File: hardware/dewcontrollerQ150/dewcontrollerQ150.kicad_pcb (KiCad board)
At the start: 2 copper layers, 54.1 x 52 mm, 17 parts, among them J1 12V Power, J2 Dew Heater, J3 SHT45 Sensor, Q1 FQP 30N06L, U2 Buck_12V_5V, U3 XIAO-ESP32-S3-DIP

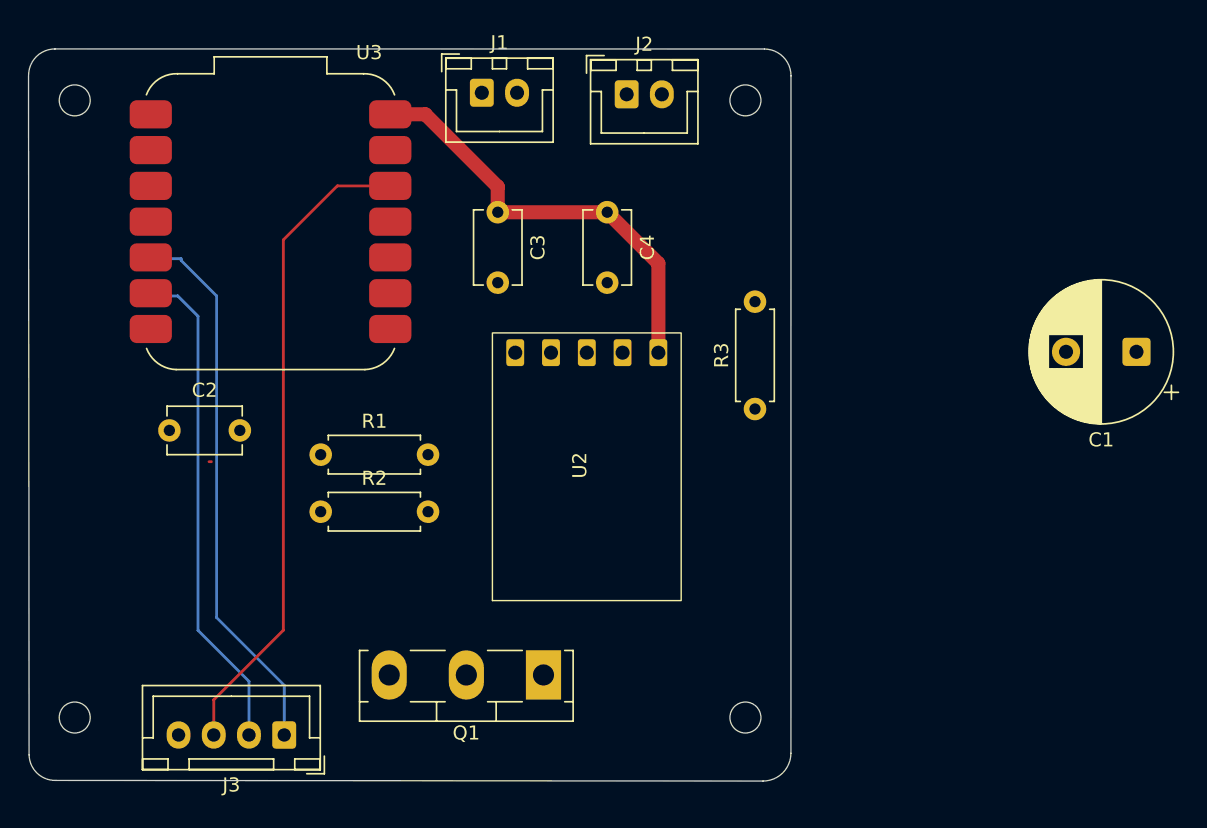
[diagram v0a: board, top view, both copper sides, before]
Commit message: v0.7 Latest CAD and KiCAD files
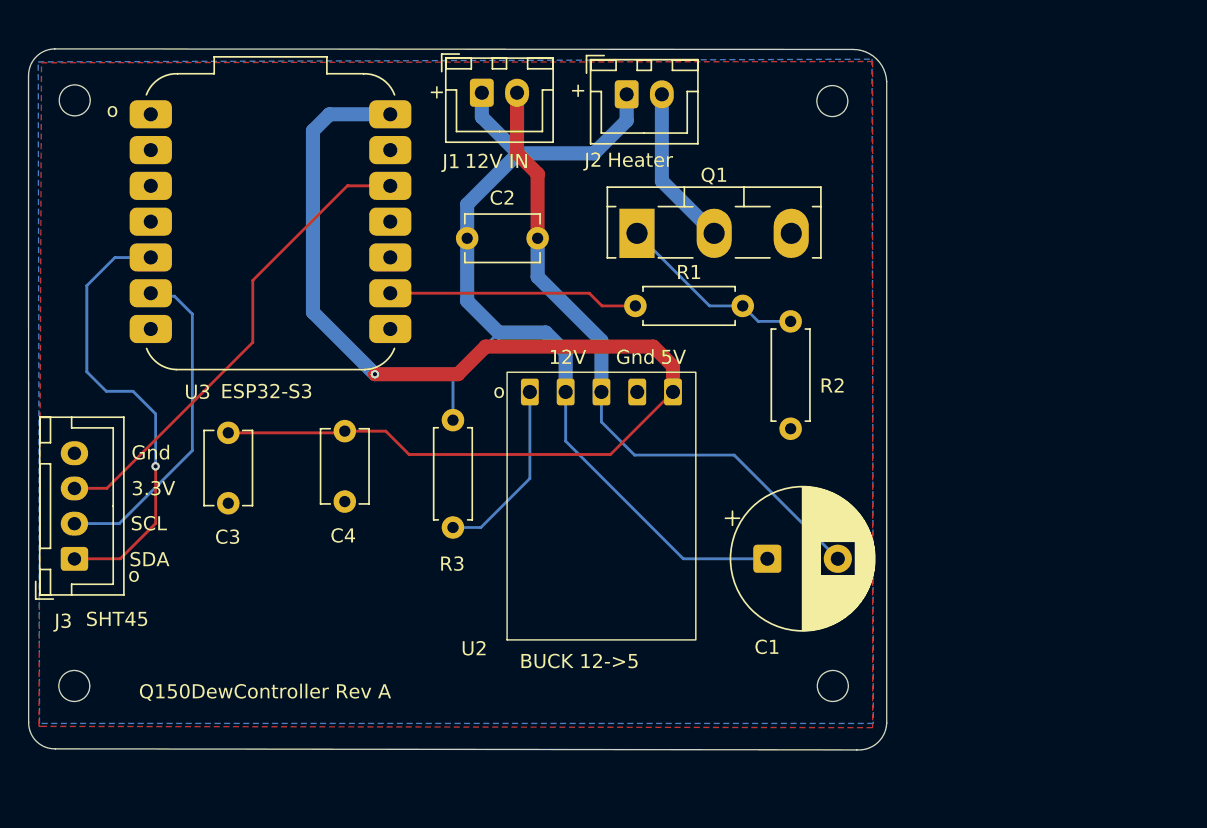
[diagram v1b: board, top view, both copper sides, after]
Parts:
- moved R2 36.0 mm to (184.1, 93.3), turned to -90 degrees
- moved Q1 32.0 mm to (173.2, 87.1), turned to 0 degrees
- moved C1 30.0 mm to (182.5, 110.2), turned to 0 degrees
- moved C2 25.2 mm to (161.2, 87.4)
- moved C3 24.7 mm to (144.2, 101.2)
- moved R1 24.7 mm to (173.1, 92.2)
- moved C4 24.3 mm to (152.5, 101.1)
- moved R3 21.5 mm to (160.1, 100.3), turned to -90 degrees
- moved J3 19.4 mm to (133.3, 110.2), turned to 90 degrees
- moved mh3 6.60 mm to (187.1, 119.2)
- moved mh2 6.17 mm to (187.1, 77.7)
- moved U2 2.98 mm to (170.7, 106.3)
- moved mh4 2.24 mm to (133.3, 119.2)
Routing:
- net +12V: track 0.00 -> 68.0 mm
- net /5V: track 31.0 -> 83.6 mm, vias 0 -> 1
- net 12V Return: track 0.00 -> 46.7 mm
- net Net-(U3-GPIO7/D8/A8/SCK): track 0.00 -> 17.8 mm
- net Net-(Q1-G): track 0.00 -> 13.5 mm
- net Net-(U2-EN): track 0.00 -> 13.0 mm
- net /3.3V: track 46.4 -> 34.0 mm
- net /SCL: track 35.2 -> 23.7 mm
- net /-Heater: track 0.00 -> 11.4 mm
- net /SDA: track 39.0 -> 32.4 mm, vias 0 -> 1
- added copper zone on B.Cu, net GND
- added copper zone on F.Cu, net GND
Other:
- board size 54.1 x 52 mm -> 60.9 x 49.8 mm
- board text added: "+"
- board text added: "12V"
- board text added: "12V IN"
- board text added: "3.3V"
- board text added: "5V"
- board text added: "BUCK 12->5"
- board text added: "ESP32-S3"
- board text added: "Gnd"
- board text added: "Heater"
- board text added: "Q150DewController Rev A"
- board text added: "SCL"
- board text added: "SDA"
- board text added: "SHT45"
- board text added: "o"
